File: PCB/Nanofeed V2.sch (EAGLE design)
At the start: 12 parts, among them J100 JST-PH_2-PIN_HEADER, J102 JST-PH_2-PIN_HEADER, J103 JST-PH_2-PIN_HEADER, J104 JST-PH_4-PIN_HEADER, J6 A4988

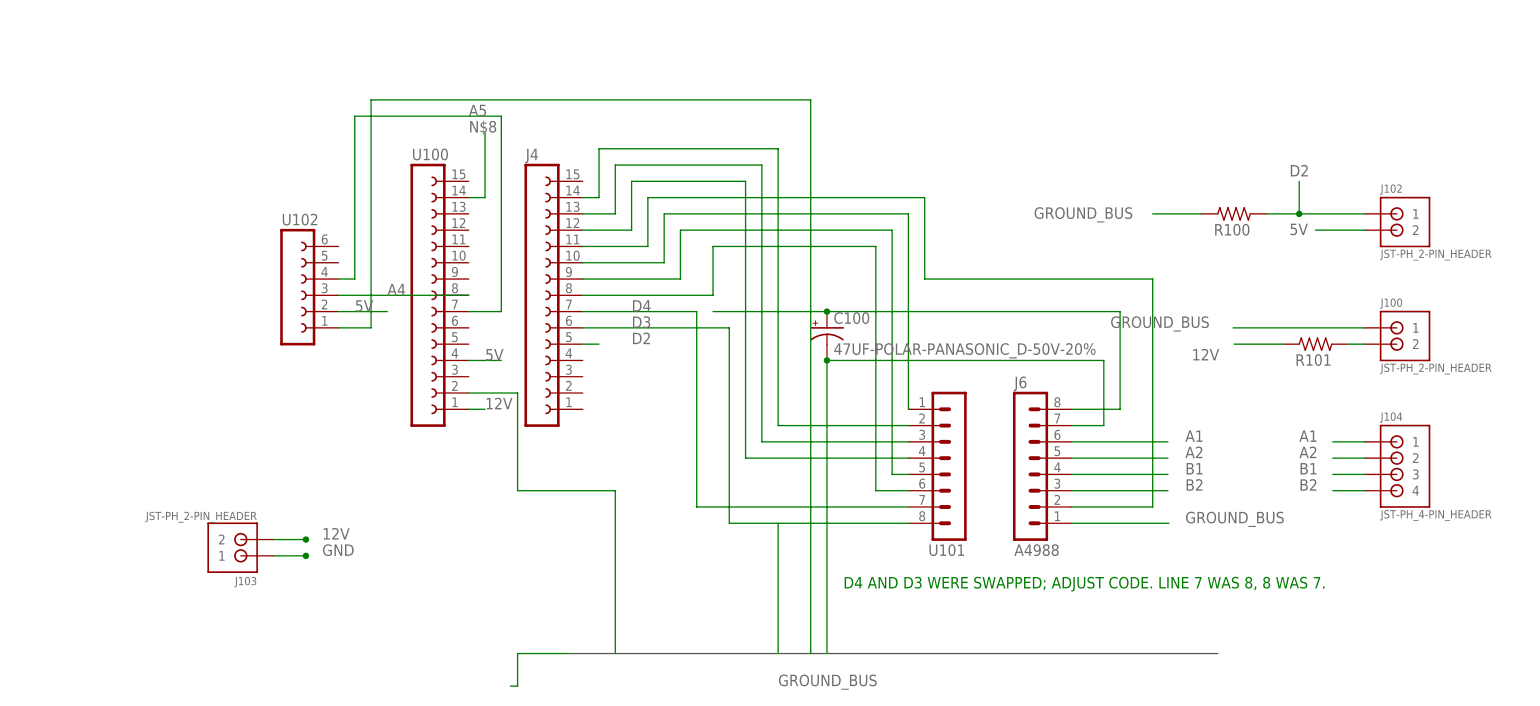
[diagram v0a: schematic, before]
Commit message: Add files via upload
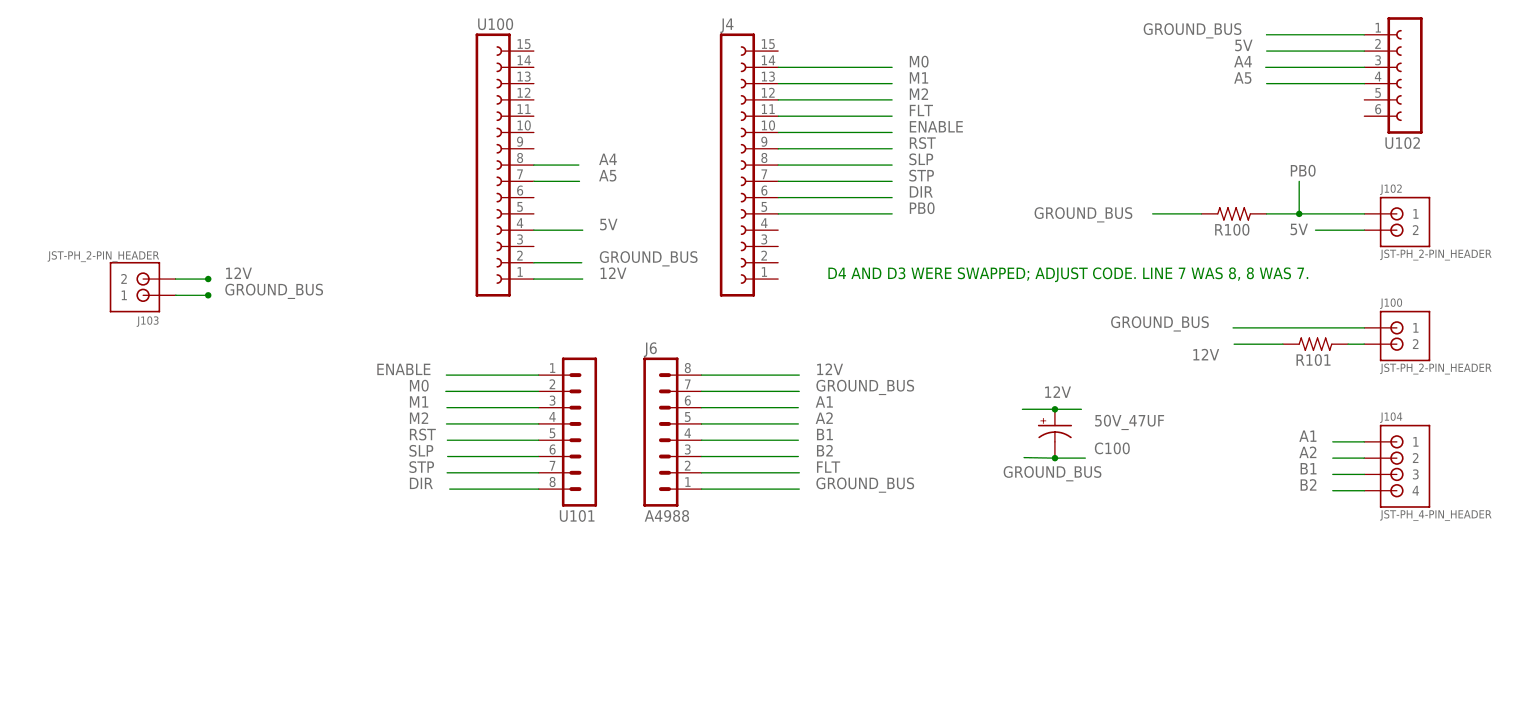
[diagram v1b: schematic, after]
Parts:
- C100: value 47UF-POLAR-PANASONIC_D-50V-20% -> 50V_47UF
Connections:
- net D2 renamed PB0
- net D3 renamed DIR
- net D4 renamed STP
- net N$1 renamed SLP
- net N$2 renamed RST
- net N$3 renamed FLT
- net N$4 renamed ENABLE
- net N$6 renamed M2
- net N$7 renamed M1
- net N$9 renamed M0
- removed net GND: J103.1
- removed net N$8: U100.14
- new net N$4: J6.7
- net GROUND_BUS: now also J103.1; no longer J6.7
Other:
- moved on the sheet: C100, J103, J4, J6, U100, U101, U102
